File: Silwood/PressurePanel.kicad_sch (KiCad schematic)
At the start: 10 parts

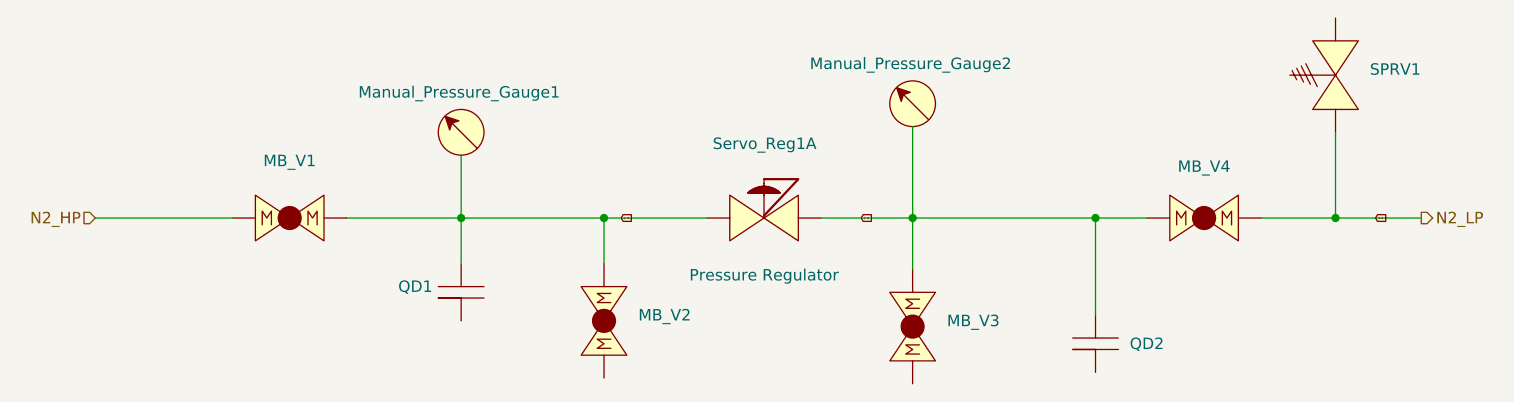
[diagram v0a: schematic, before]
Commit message: silwood upgrade
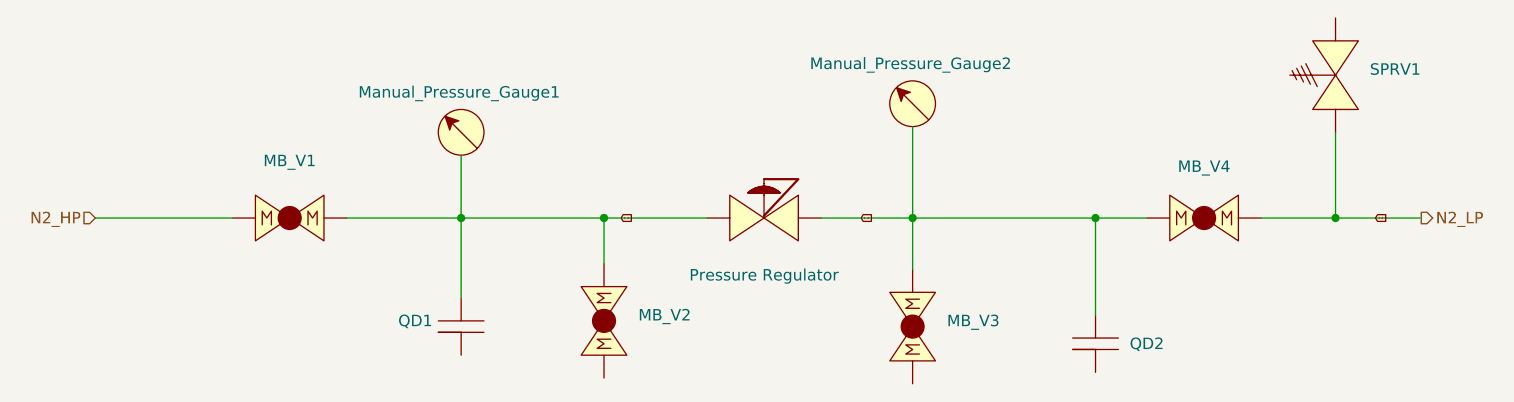
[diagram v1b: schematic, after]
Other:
- moved on the sheet: QD1
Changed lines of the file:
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@@
 	(wire
 		(pts
-			(xy 84.455 88.265) (xy 84.455 83.185)
+			(xy 84.455 92.075) (xy 84.455 83.185)
 		)
 		(stroke
@@
 					(size 1.27 1.27)
 				)
+				(hide yes)
 			)
 		)
@@
 		(lib_name "Quick_Disconnect_1")
 		(lib_id "PID_symbols:Quick_Disconnect")
-		(at 84.455 92.075 90)
+		(at 84.455 95.885 90)
 		(unit 1)
 		(exclude_from_sim no)
@@
 		(fields_autoplaced yes)
 		(property "Reference" "QD1"
-			(at 81.28 90.8049 90)
+			(at 81.28 94.6149 90)
 			(effects
 				(font
@@
 		)
 		(property "Value" "~"
-			(at 81.28 92.71 90)
+			(at 81.28 96.52 90)
 			(effects
 				(font
@@
 		)
 		(property "Footprint" ""
-			(at 84.455 92.075 0)
-			(effects
-				(font
-					(size 1.27 1.27)
-				)
-				(hide yes)
-			)
-		)
-		(property "Datasheet" ""
-			(at 84.455 92.075 0)
+			(at 84.455 95.885 0)
+			(effects
+				(font
+					(size 1.27 1.27)
+				)
+				(hide yes)
+			)
+		)
+		(property "Datasheet" ""
+			(at 84.455 95.885 0)
 			(effects
 				(font
@@
 		)
 		(property "Description" ""
-			(at 84.455 92.075 0)
-			(effects
-				(font
+			(at 84.455 95.885 0)
+			(effects
+				(font
